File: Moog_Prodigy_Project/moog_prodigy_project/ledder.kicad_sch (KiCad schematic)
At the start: 72 parts, among them J6 NJ2FD-V, Q10 CA3046, Q11 BC327, Q14 BC550C, Q15 BC550C, Q16 BC550C, Q17 BC550C, Q18 BC550C, Q19 BC550C, Q8 BC556, Q9 CA3046, SW11 FILTER MODE, U1 LT1469, U15 LT1469, U16 LT1228, U17 NE5532

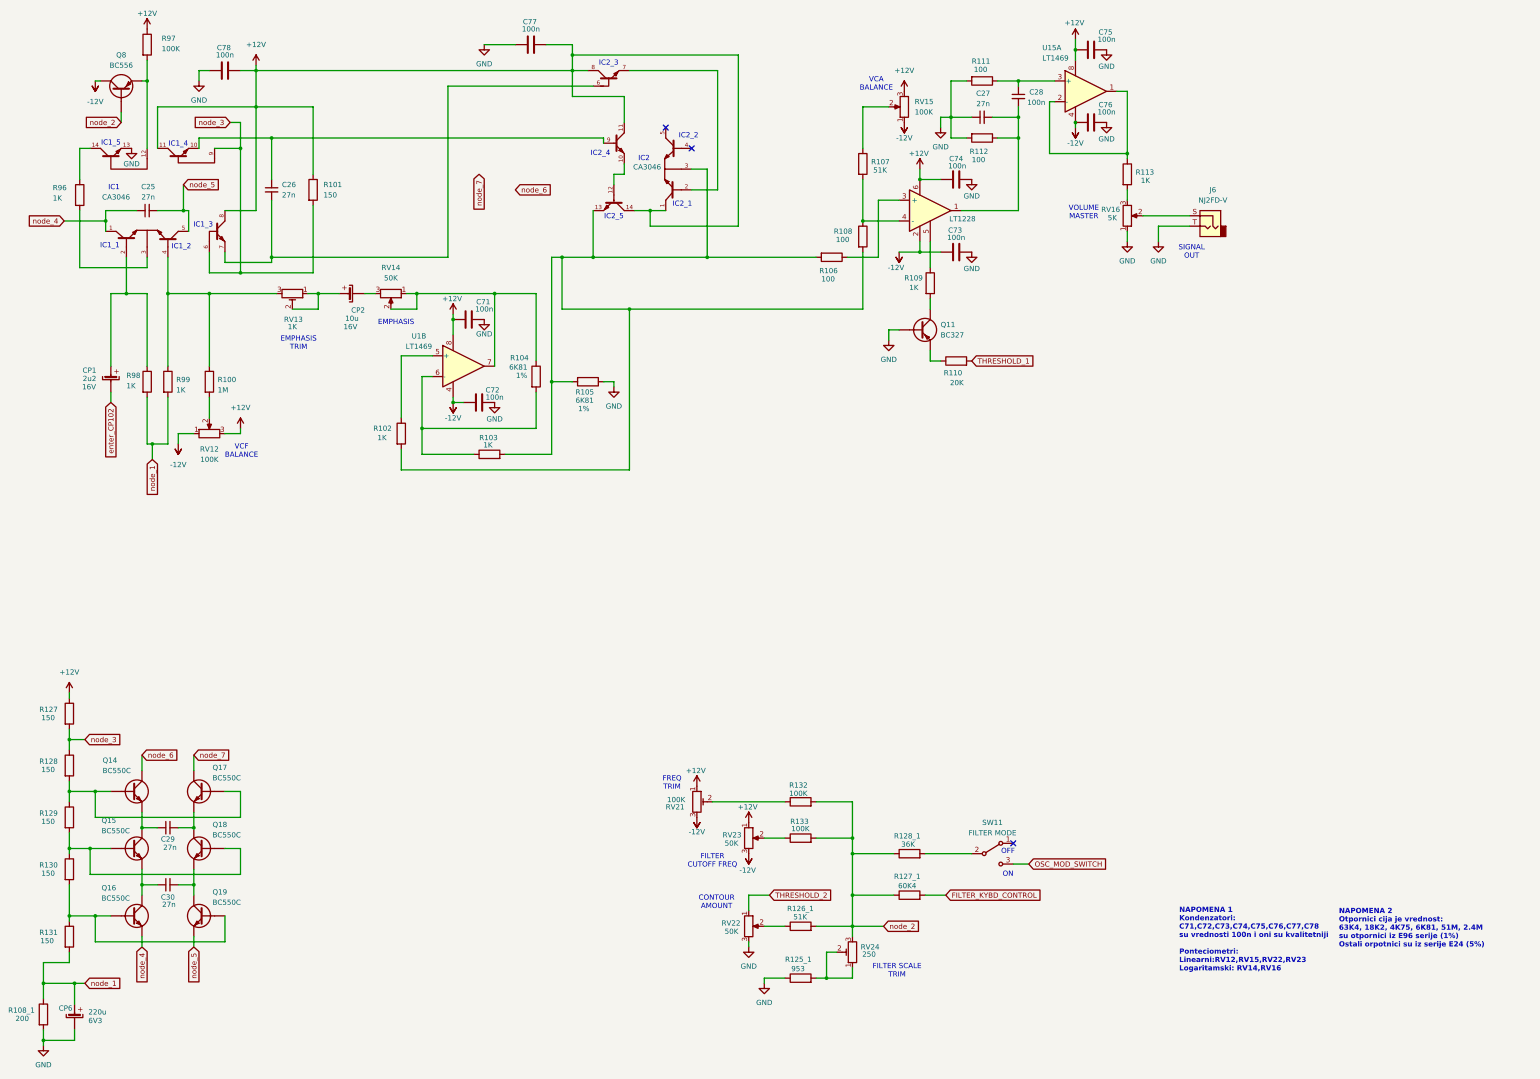
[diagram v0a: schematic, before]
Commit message: 04.07.2026 Dodati tolerancije, E94, prosiriti spisak
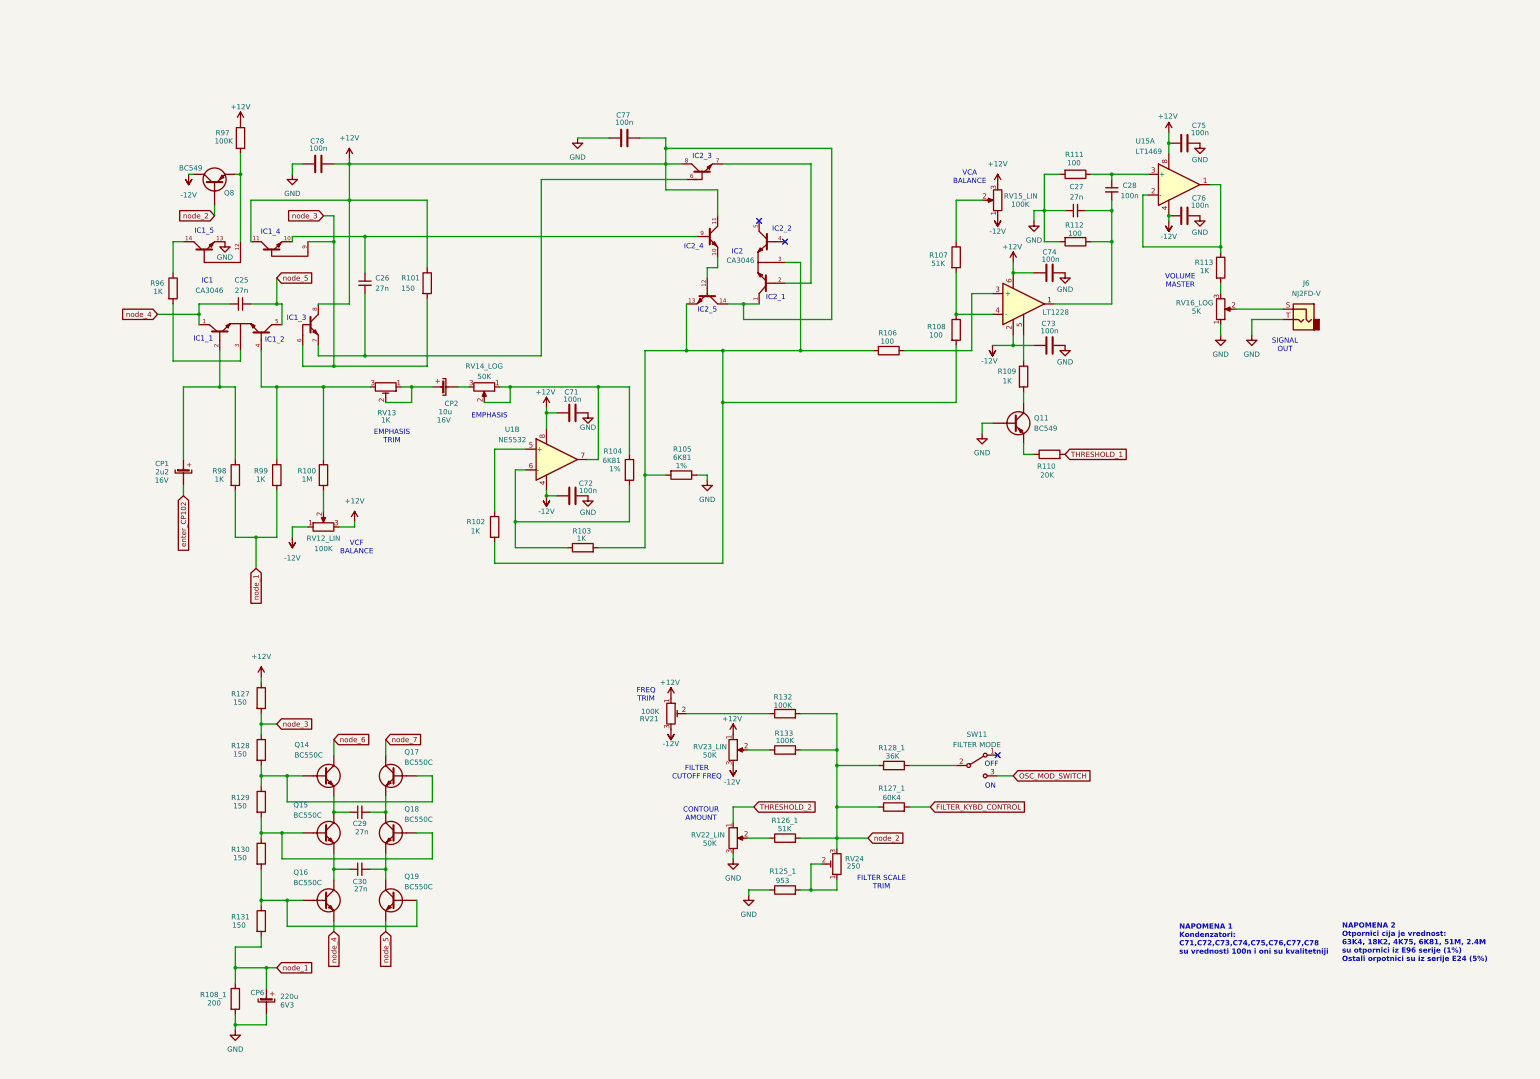
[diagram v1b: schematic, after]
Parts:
- Q11: value BC327 -> BC549
- Q8: value BC556 -> BC549
- U1: value LT1469 -> NE5532
- renumbered RV12 to RV12_LIN, RV14 to RV14_LOG, RV15 to RV15_LIN, RV16 to RV16_LOG, RV22 to RV22_LIN, RV23 to RV23_LIN
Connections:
- new net: C29.2, Q17. (E), Q18. (E)
- new net: C29.1, Q14. (E), Q15. (E)
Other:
- note added: "NAPOMENA 1 Kondenzatori: C71,C72,C73,C74,C75,C76,C77,C78 su vrednosti 100n i oni su kvalitetniji"
- note removed: "NAPOMENA 1 Kondenzatori: C71,C72,C73,C74,C75,C76,C77,C78 su vrednosti 100n i oni su kvalitetniji Ponteciometri: Linearni:RV12,RV15,RV22,RV23 Logaritamski: RV14,RV16"
- moved on the sheet: C25, C26, C27, C28, C29, C30, C71, C72, C73, C74, C75, C76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
